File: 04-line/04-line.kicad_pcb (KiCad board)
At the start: 2 copper layers, 80 x 65 mm, 83 parts, among them J1 ST-LINK, J3 ToMAIN, J4 WRITER CONN, U24 STM32F446RETx

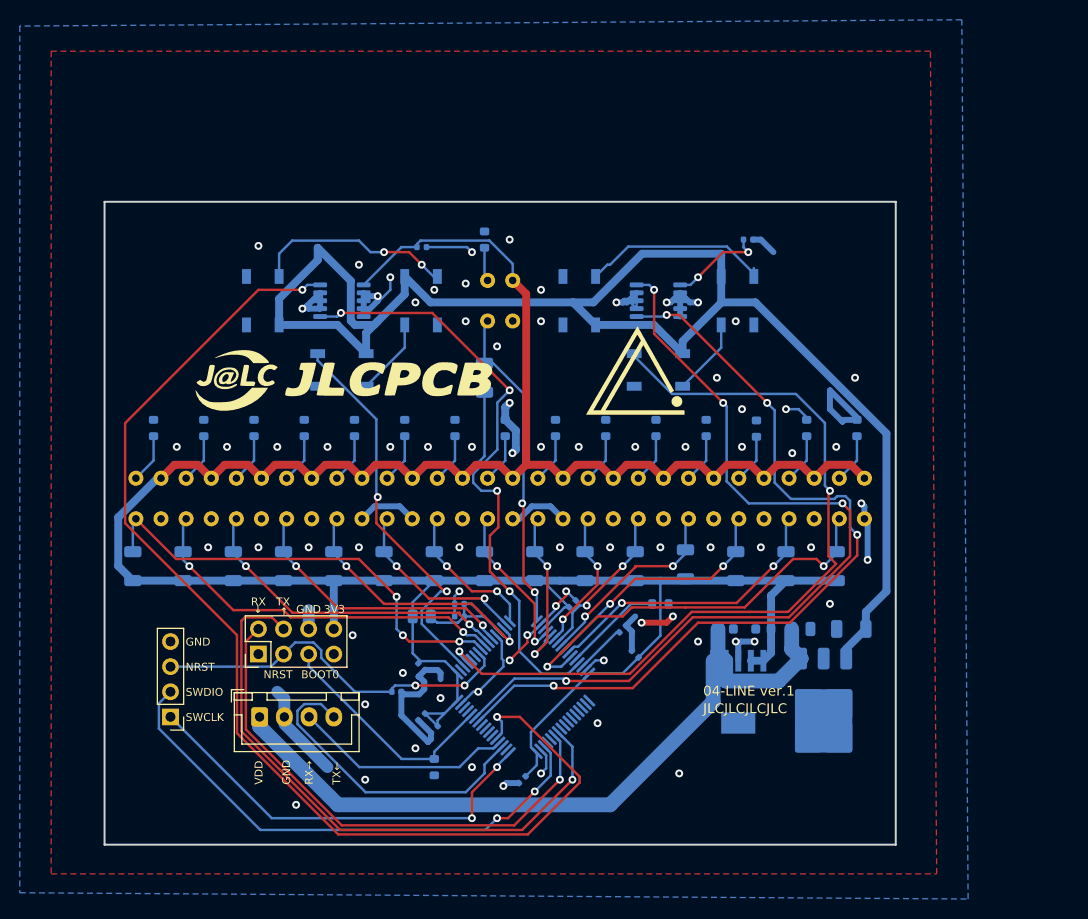
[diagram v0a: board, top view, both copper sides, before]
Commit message: いっぱい増えた
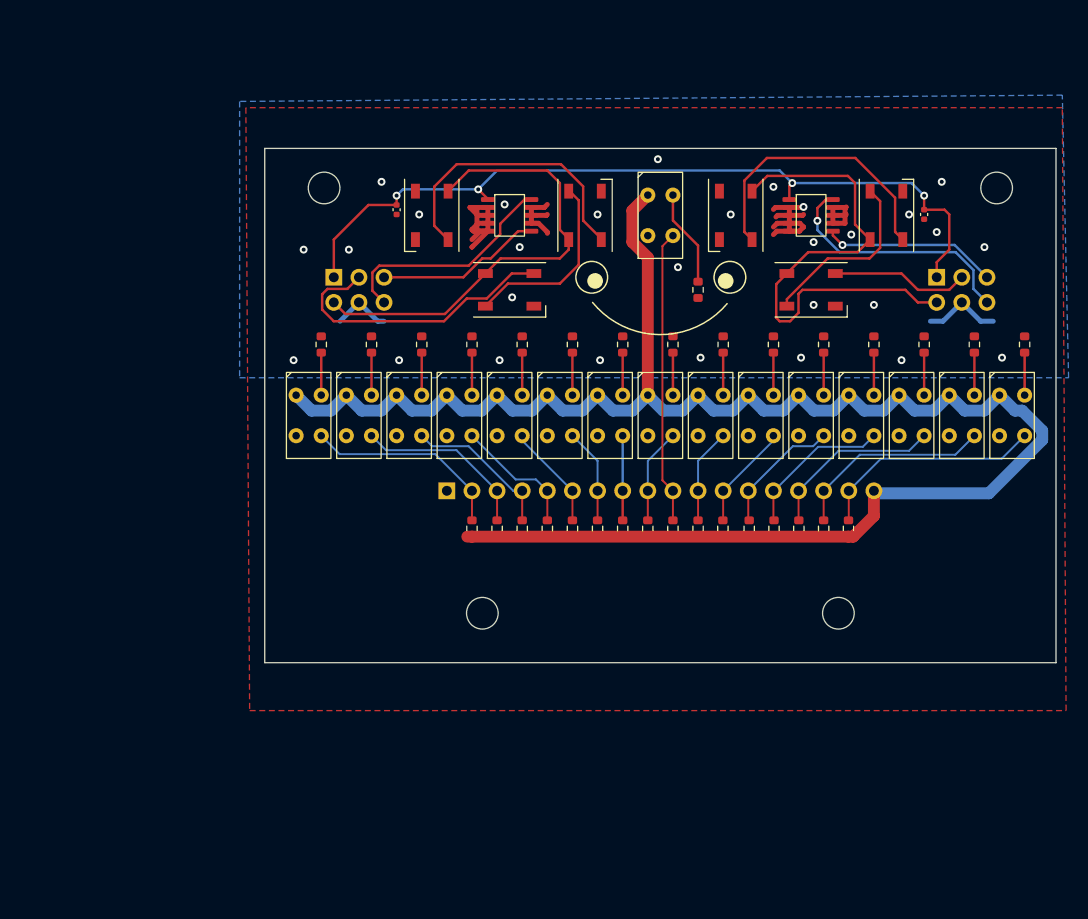
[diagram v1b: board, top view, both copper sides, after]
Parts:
- removed C1, C11, C12, C13, C15, C4, C5: 100n, Capacitor_SMD:C_0402_1005Metric
- removed C10: 100u, Capacitor_SMD:C_1206_3216Metric
- removed C14, C2: 4.7u, Capacitor_SMD:C_0402_1005Metric
- removed C16: 1u, Capacitor_SMD:C_0402_1005Metric
- removed C7, C8: 10u, Capacitor_SMD:C_0603_1608Metric
- removed C9: 0.33u, Capacitor_SMD:C_0805_2012Metric
- removed FB1: FerriteBead, Resistor_SMD:R_0805_2012Metric
- removed J4: WRITER CONN, Connector_PinHeader_2.54mm:PinHeader_2x04_P2.54mm_Vertical
- removed R26, R37: 10k, Resistor_SMD:R_0603_1608Metric
- removed U24: STM32F446RETx, Package_QFP:LQFP-64_10x10mm_P0.5mm
- removed U27: ~, Package_TO_SOT_SMD:SOT-223-6
- removed U28: ~, Package_TO_SOT_SMD:TO-252-3_TabPin2
- added J2: CS_R, Connector_PinHeader_2.54mm:PinHeader_2x03_P2.54mm_Vertical, B.Cu at (68.6, 87.6)
- added REF**: MountingHole_3.2mm_M3, MountingHole:MountingHole_3.2mm_M3, F.Cu at (67.6, 78.6)
- added REF**: MountingHole_3.2mm_M3, MountingHole:MountingHole_3.2mm_M3, F.Cu at (135.6, 78.6)
- added REF**: MountingHole_3.2mm_M3, MountingHole:MountingHole_3.2mm_M3, F.Cu at (119.6, 121.6)
- added REF**: MountingHole_3.2mm_M3, MountingHole:MountingHole_3.2mm_M3, F.Cu at (83.6, 121.6)
- C3, C6, D1, D2, D4, D5, D6, D8, U10, U12, U13, U14, U15, U16, U17, U18, U2, U25, U26, U3, U4, U5, U6, U7, U8, U9: moved to F.Cu
- G*** (x2): moved to B.Cu
- J1: value ST-LINK -> Conn_01x18; footprint Connector_PinHeader_2.54mm:PinHeader_1x04_P2.54mm_Vertical -> Connector_PinHeader_2.54mm:PinHeader_1x18_P2.54mm_Vertical; moved to B.Cu
- J3: value ToMAIN -> CS_L; footprint Connector_JST:JST_XH_B4B-XH-A_1x04_P2.50mm_Vertical -> Connector_PinHeader_2.54mm:PinHeader_2x03_P2.54mm_Vertical; moved to B.Cu
- R1, R19, R2, R20, R21, R22, R23, R24, R25, R3, R4, R5, R6, R7, R8, R9: value 105 -> 120; moved to F.Cu
- R10, R11, R12, R13, R14, R15, R16, R17, R18, R28, R29, R30, R31, R32, R33, R34: footprint Resistor_SMD:R_1206_3216Metric -> Resistor_SMD:R_0603_1608Metric; moved to F.Cu
- moved J3 81.6 mm to (129.5, 87.6), turned to -90 degrees
- moved C3 50.9 mm to (128.3, 81.3), turned to -90 degrees
- moved U25 48.2 mm to (116.8, 81.4), turned to 0 degrees
- moved G*** 42.3 mm to (111.3, 90.7), turned to 180 degrees
- moved J1 36.1 mm to (80.0, 109.2), turned to -90 degrees
- moved C6 35.7 mm to (74.9, 80.8), turned to -90 degrees
- moved R16 34.5 mm to (82.5, 113.0)
- moved R15 32.0 mm to (85.1, 113.0)
- moved R14 29.5 mm to (87.6, 113.0)
- moved R13 26.9 mm to (90.2, 113.0)
- moved R12 24.4 mm to (92.7, 113.0)
- moved R18 24.4 mm to (102.9, 113.0)
- moved R9 22.2 mm to (105.4, 88.9), turned to -90 degrees
- moved R11 21.9 mm to (95.2, 113.0)
- moved R10 19.4 mm to (97.8, 113.0)
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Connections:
- C3 pad 1: +3V3 -> SENSER_3V3
- C6 pad 1: +3V3 -> SENSER_3V3
- D1 pad 1: +5V -> 5V_LED
- D2 pad 1: +5V -> 5V_LED
- D4 pad 1: +5V -> 5V_LED
- D5 pad 1: +5V -> 5V_LED
- D6 pad 1: +5V -> 5V_LED
- D8 pad 1: +5V -> 5V_LED
- J1 pad 1: SWCLK -> GND
- J1 pad 2: SWDIO -> photo_L_7
- J1 pad 3: NRST -> photo_L_6
- J1 pad 4: GND -> photo_L_5
- J3 pad 1: VDD -> SENSER_3V3
- J3 pad 2: GND -> 5V_LED
- J3 pad 3: UART3_RX -> LED_L
- J3 pad 4: UART3_TX -> GND
- U25 pad 1: +3V3 -> SENSER_3V3
- U26 pad 1: +3V3 -> SENSER_3V3
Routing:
- net +5V: track 147.4 -> 0.00 mm
- net +3V3: track 307.9 -> 181.0 mm, vias 2 -> 0
- net 5V_LED: track 0.00 -> 98.5 mm
- net I2C2_SDA: track 116.7 -> 25.4 mm, vias 2 -> 1
- net GND: track 145.7 -> 60.0 mm, vias 76 -> 29
- net SENSER_3V3: track 0.00 -> 82.3 mm, vias 0 -> 4
- net VDD: track 76.1 -> 0.00 mm
- net I2C1_SCL: track 85.2 -> 16.8 mm, vias 4 -> 0
- net LED_L: track 82.3 -> 14.0 mm, vias 2 -> 0
- net I2C1_SDA: track 87.6 -> 23.3 mm, vias 4 -> 0
- net UART1_TX: track 61.2 -> 0.00 mm, vias 1 -> 0
- net SWDIO: track 53.6 -> 0.00 mm, vias 2 -> 0
- net UART1_RX: track 53.1 -> 0.00 mm, vias 1 -> 0
- net I2C2_SCL: track 61.4 -> 17.8 mm, vias 4 -> 1
- net SWCLK: track 42.9 -> 0.00 mm, vias 2 -> 0
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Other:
- board size 80 x 65 mm -> 80 x 52 mm
- board text removed: "04-LINE ver.1"
- board text removed: "1"
- board text removed: "3V3"
- board text removed: "3V3 REG"
- board text removed: "5V REG"
- board text removed: "BOOT0"
- board text removed: "GND"
- board text removed: "JLCJLCJLCJLC"
- board text removed: "NRST"
- board text removed: "RX"
- board text removed: "RX→"
- board text removed: "SWCLK"
- board text removed: "SWDIO"
- board text removed: "TX"
- board text removed: "TX←"
- board text removed: "VDD"
- board text removed: "↓"
